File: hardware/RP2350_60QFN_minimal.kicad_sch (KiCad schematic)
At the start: 37 parts, among them J4 SM03B-SRSS-TB, J5 4677, SW1 SW_Push, SW2 SW_Push, U1 RP2350_60QFN, U3 W25Q128JVS, Y1 ABM8-272-T3

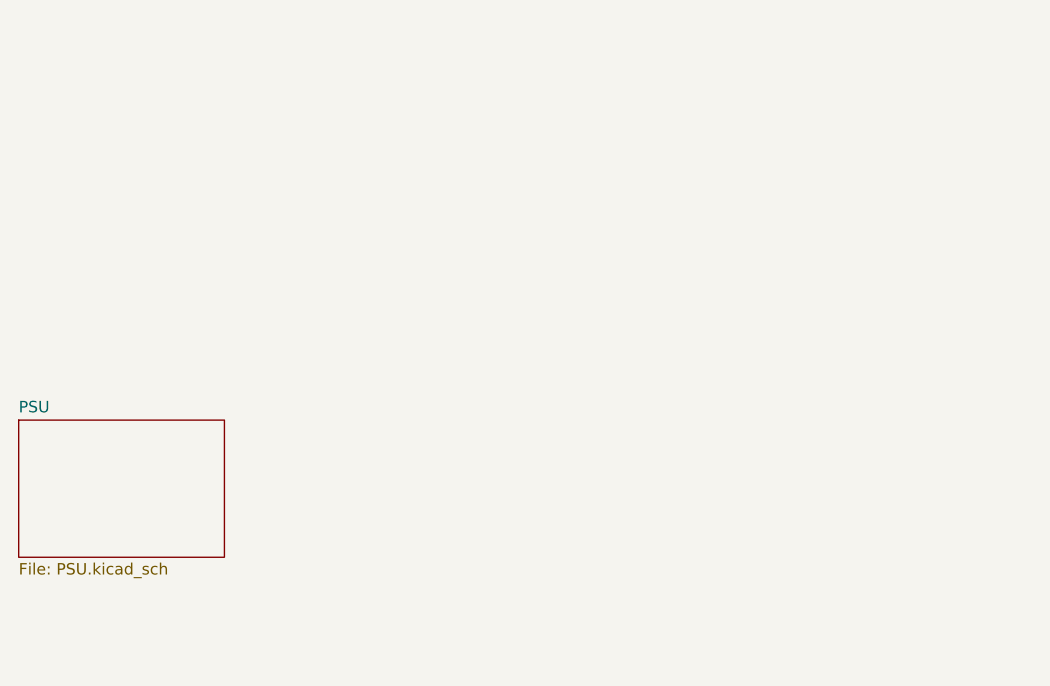
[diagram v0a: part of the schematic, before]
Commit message: Up to date
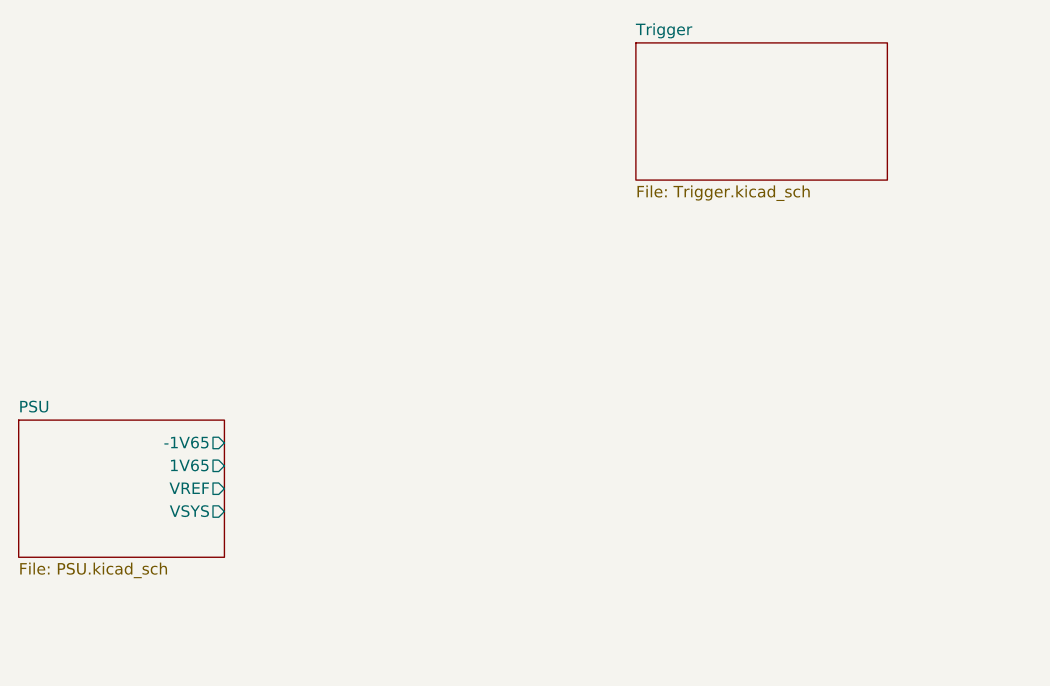
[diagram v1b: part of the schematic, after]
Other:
- added sheet Trigger (Trigger.kicad_sch)
- sheet PSU ports: added -1V65, 1V65, VREF, VSYS; removed none
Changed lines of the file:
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@@
+			)
+		)
+		(pin "-1V65" output
+			(at 143.51 88.9 0)
+			(effects
+				(font
+					(size 1.27 1.27)
+				)
+				(justify right)
+			)
+		)
+		(pin "1V65" output
+			(at 143.51 91.44 0)
+			(effects
+				(font
+					(size 1.27 1.27)
+				)
+				(justify right)
+			)
+		)
+		(pin "VREF" output
+			(at 143.51 93.98 0)
+			(effects
+				(font
+					(size 1.27 1.27)
+				)
+				(justify right)
+			)
+		)
+		(pin "VSYS" output
+			(at 143.51 96.52 0)
+			(effects
+				(font
+					(size 1.27 1.27)
+				)
+				(justify right)
 			)
 		)
@@
 				)
 			)
+		)
+	)
+	(sheet
+		(at 189.23 44.45)
+		(size 27.94 15.24)
+		(exclude_from_sim no)
+		(in_bom yes)
+		(on_board yes)
+		(dnp no)
+		(fields_autoplaced yes)
+		(stroke
+			(width 0.1524)
+			(type solid)
+		)
+		(fill
+			(color 0 0 0 0.0000)
+		)
+		(property "Sheetname" "Trigger"
+			(at 189.23 43.7384 0)
+			(effects
+				(font
+					(size 1.27 1.27)
+				)
+				(justify left bottom)
+			)
+		)
+		(property "Sheetfile" "Trigger.kicad_sch"
+			(at 189.23 60.2746 0)
+			(effects
+				(font
+					(size 1.27 1.27)
+				)
+				(justify left top)
+			)
+		)
+		(instances
+			(project "RP2350_60QFN_minimal"
+				(path "/94683f5c-9cd9-448e-be96-9792537b5cb8"
+					(page "4")
+				)
+			)
